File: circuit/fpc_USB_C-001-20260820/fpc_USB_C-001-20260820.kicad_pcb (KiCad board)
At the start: 2 copper layers, 2 parts, among them P1 USB_C_Plug, P2 USB_C_Plug

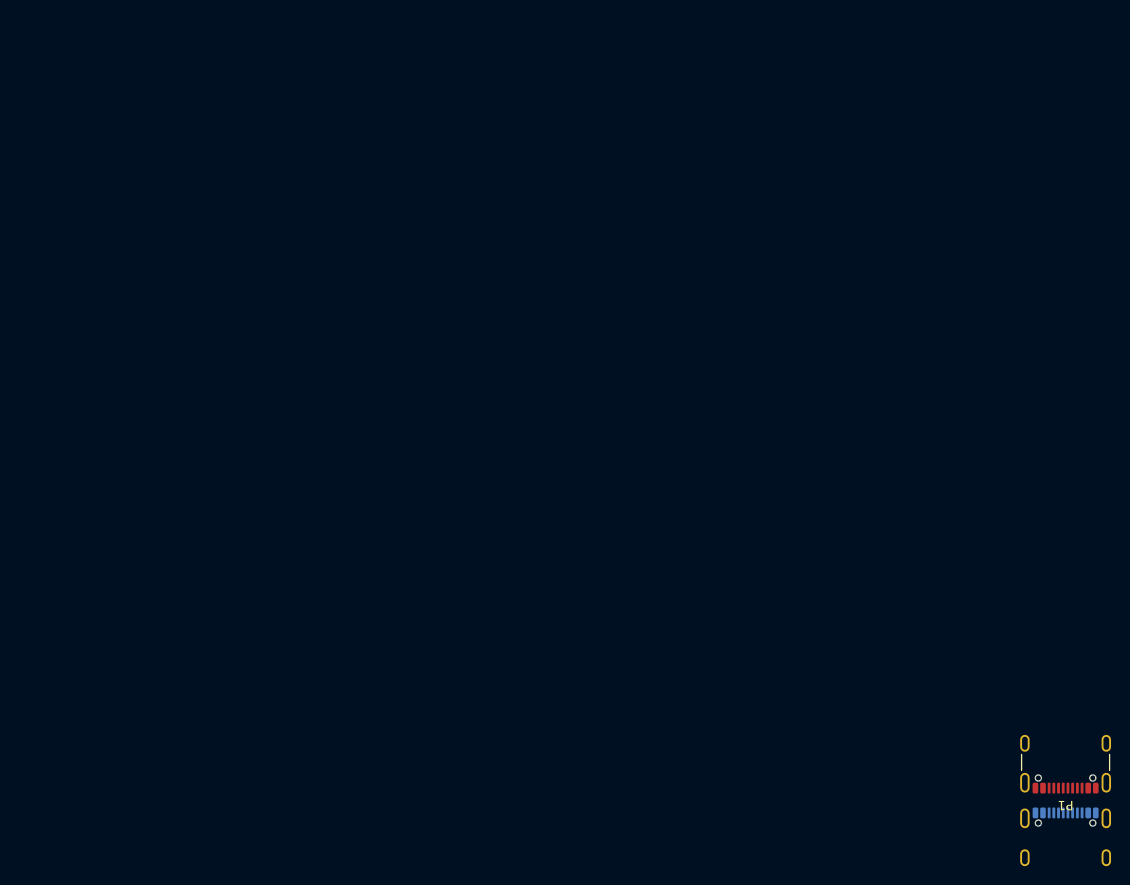
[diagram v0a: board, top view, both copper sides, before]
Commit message: Update カメラ用のUSB-CのFPCケーブルを作ろうとした
フットプリントどうしよ
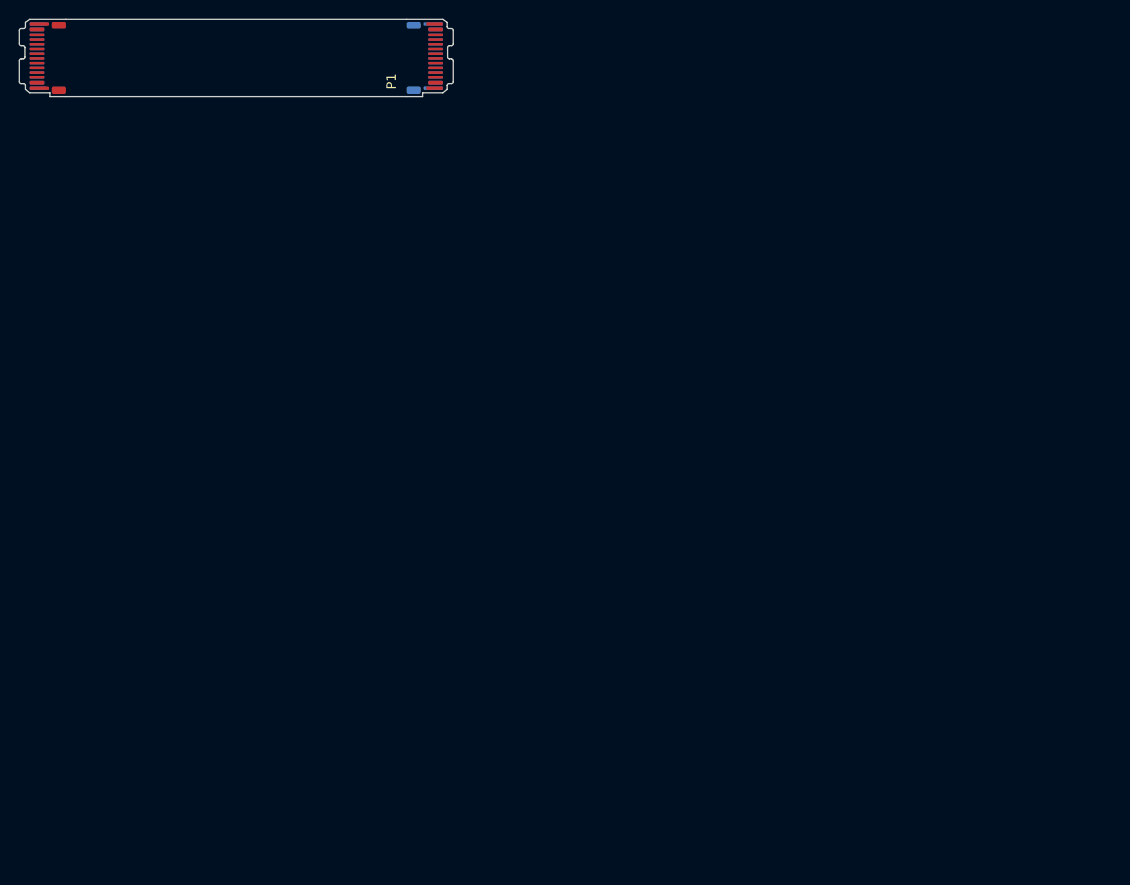
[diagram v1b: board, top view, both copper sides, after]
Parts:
- P1, P2: footprint Connector_USB:USB_C_Receptacle_GCT_USB4105-xx-A_16P_TopMnt_Horizontal -> Connector_USB:USB_C_Plug_JAE_DX07P024AJ1
- moved P2 136.8 mm to (0.00, 0.00), turned to 90 degrees
- moved P1 100.5 mm to (40.0, 0.00), turned to 90 degrees
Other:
- board outline added: 36.2 x 8.2 mm
